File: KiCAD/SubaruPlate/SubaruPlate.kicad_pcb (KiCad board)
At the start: 2 copper layers, 140 x 140 mm, 24 parts, among them J1 DF51A-4P-2DSA, J2 B3B-XH-A(LF)(SN), U1 LPS28DFW, U3 MCP2515-xSO, U4 MCP2562-E-SN, U5 XIAO-RP2040-DIP, Y1 8MHz

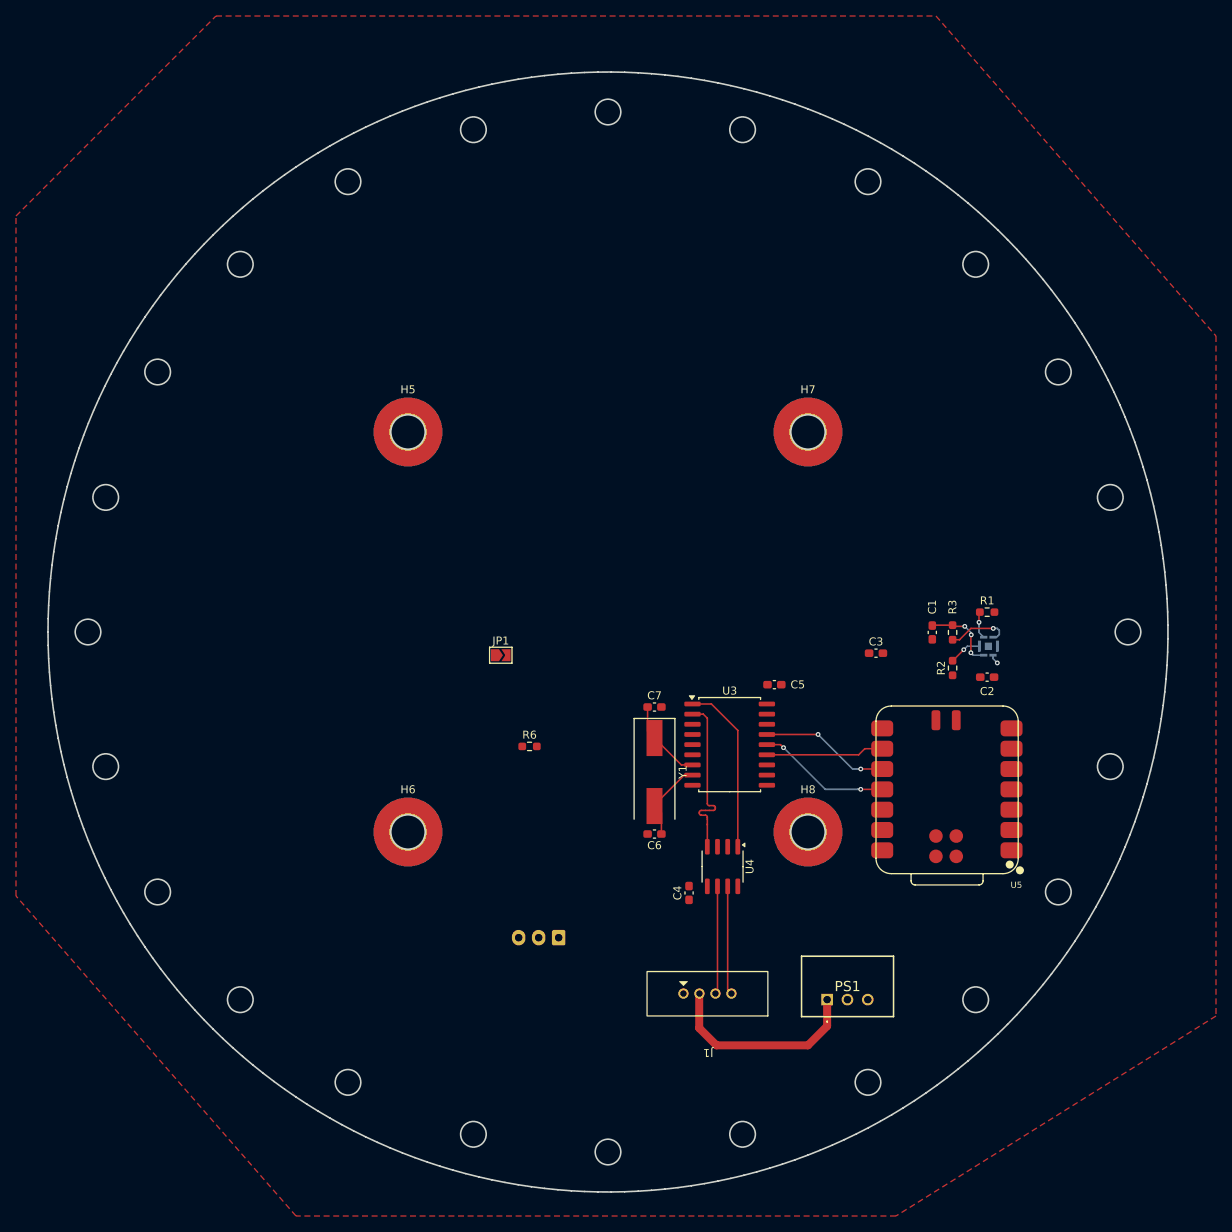
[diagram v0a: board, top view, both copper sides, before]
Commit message: 後は最終確認
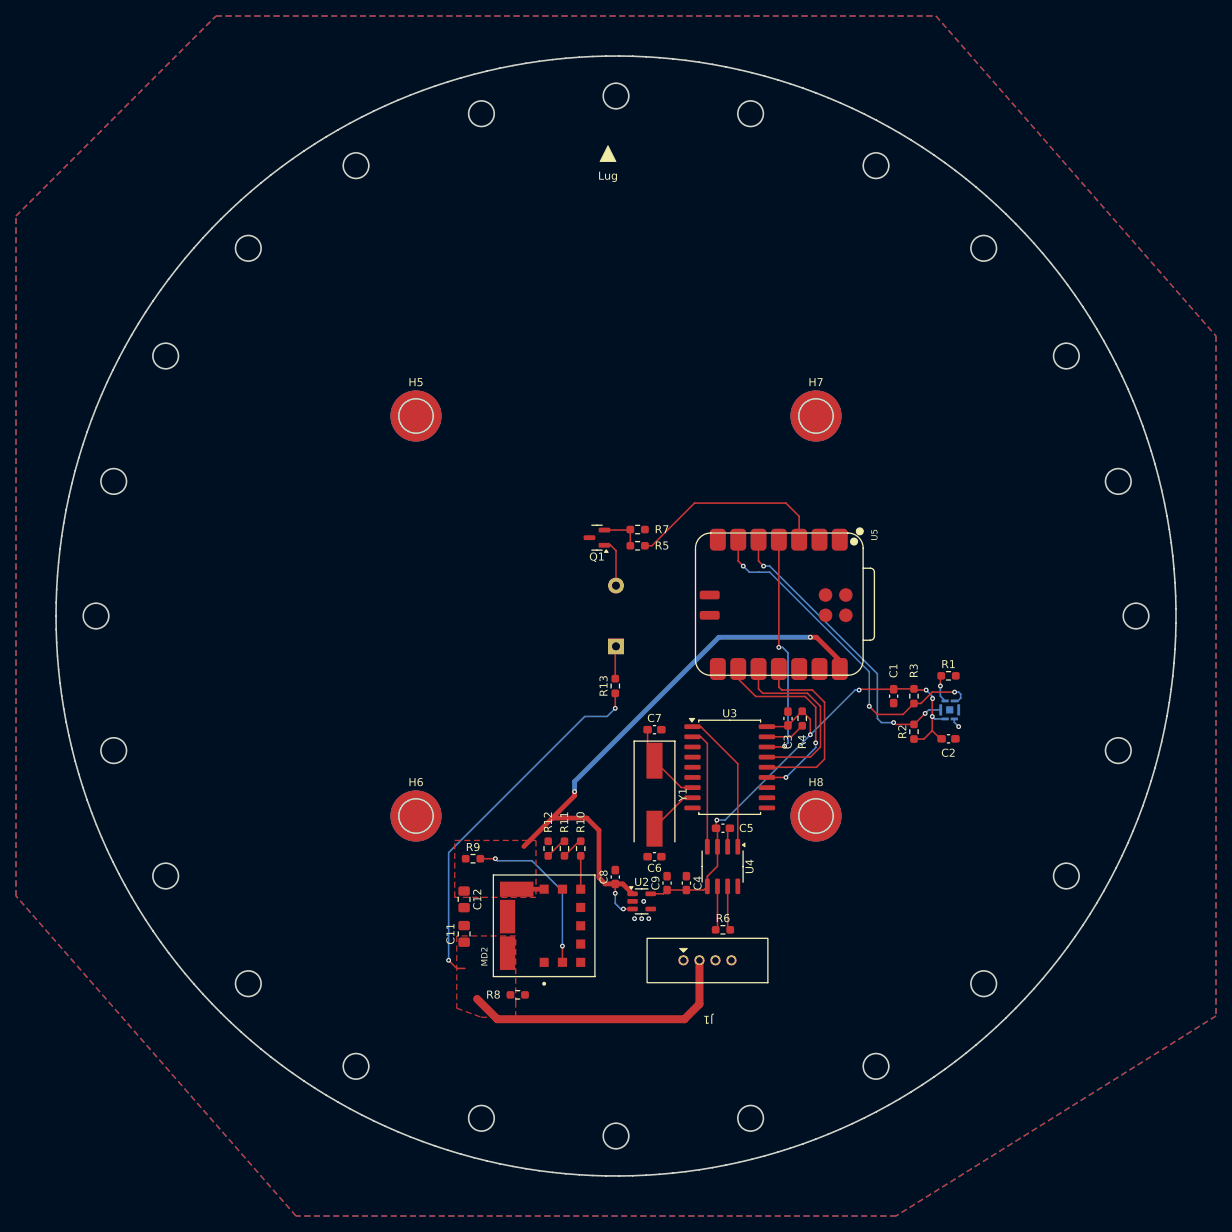
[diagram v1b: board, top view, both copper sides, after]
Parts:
- removed J2: B3B-XH-A(LF)(SN), Connector_JST:JST_XH_B3B-XH-A_1x03_P2.50mm_Vertical
- removed JP1: Jumper_2_Open, Jumper:SolderJumper-2_P1.3mm_Open_TrianglePad1.0x1.5mm
- removed PS1: M78AR05-0.5, TSRP_IC:M78AR03305
- added BZ1: Buzzer, Buzzer_Beeper:Buzzer_12x9.5RM7.6, B.Cu at (150.0, 103.8)
- added C11: 22u, Capacitor_SMD:C_0805_2012Metric_Pad1.18x1.45mm_HandSolder, F.Cu at (131.0, 139.7)
- added C12: 10u, Capacitor_SMD:C_0805_2012Metric_Pad1.18x1.45mm_HandSolder, F.Cu at (131.0, 135.4)
- added C8: 1u, Capacitor_SMD:C_0603_1608Metric_Pad1.08x0.95mm_HandSolder, F.Cu at (149.9, 132.6)
- added C9: 1u, Capacitor_SMD:C_0603_1608Metric_Pad1.08x0.95mm_HandSolder, F.Cu at (156.4, 133.4)
- added MD2: OKL-T_6-W12N-C, TSRP_IC:MURATA_OKL-T-6-W12N-C_0, F.Cu at (141.0, 138.7)
- added Q1: NMOS, Package_TO_SOT_SMD:SOT-23, F.Cu at (147.6, 90.2)
- added R10: 1k 0.1%, Resistor_SMD:R_0603_1608Metric_Pad0.98x0.95mm_HandSolder, F.Cu at (145.6, 129.1)
- added R11: 330 0.1%, Resistor_SMD:R_0603_1608Metric_Pad0.98x0.95mm_HandSolder, F.Cu at (143.6, 129.1)
- added R12: 10 0.1%, Resistor_SMD:R_0603_1608Metric_Pad0.98x0.95mm_HandSolder, F.Cu at (141.5, 129.1)
- added R13: 600, Resistor_SMD:R_0603_1608Metric_Pad0.98x0.95mm_HandSolder, F.Cu at (149.9, 108.8)
- added R4: 10K, Resistor_SMD:R_0603_1608Metric_Pad0.98x0.95mm_HandSolder, F.Cu at (173.3, 112.8)
- added R5: 750, Resistor_SMD:R_0603_1608Metric_Pad0.98x0.95mm_HandSolder, F.Cu at (152.7, 91.2)
- added R7: 10k, Resistor_SMD:R_0603_1608Metric_Pad0.98x0.95mm_HandSolder, F.Cu at (152.7, 89.2)
- added R8: 20k, Resistor_SMD:R_0603_1608Metric_Pad0.98x0.95mm_HandSolder, F.Cu at (137.7, 147.4)
- added R9: 100k, Resistor_SMD:R_0603_1608Metric_Pad0.98x0.95mm_HandSolder, F.Cu at (132.1, 130.3)
- added U2: NCV8114BSN330T1G, Package_TO_SOT_SMD:TSOT-23-5, F.Cu at (153.2, 135.7)
- H5, H6, H7, H8: footprint MountingHole:MountingHole_4.3mm_M4_Pad_TopBottom -> MountingHole:MountingHole_3.2mm_M3_Pad_TopBottom
- moved R6 33.3 mm to (163.4, 139.2)
- moved U5 31.4 mm to (170.4, 98.5), turned to -90 degrees
- moved C5 19.1 mm to (163.4, 126.5)
- moved C3 13.7 mm to (171.5, 112.8), turned to 90 degrees
- moved R1 9.31 mm to (191.6, 107.5)
- moved C1 9.31 mm to (184.7, 110.0)
- moved R2 9.31 mm to (187.2, 114.5)
- moved R3 9.31 mm to (187.2, 110.0)
- moved U1 9.31 mm to (191.7, 111.7)
- moved C2 9.10 mm to (191.6, 115.4)
- moved J1 4.15 mm to (161.4, 140.4)
- moved C6 2.83 mm to (154.8, 130.1)
- moved C7 2.83 mm to (154.8, 114.2)
- moved U3 2.83 mm to (164.2, 118.9)
- moved Y1 2.83 mm to (154.8, 122.3)
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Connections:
- R6 pad 2: Net-(JP1-B) -> CAN_H
- U5 pad 12: +3.3V -> unconnected-(U5-3V3-Pad12)
- U5 pad 3: unconnected-(U5-GPIO28/ADC2/A2-Pad3) -> Buzzer
- U5 pad 4: unconnected-(U5-GPIO29/ADC3/A3-Pad4) -> SPI_CS_MCP2515
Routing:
- net +5V: track 0.00 -> 79.6 mm, vias 0 -> 4
- net +3.3V: track 9.54 -> 69.4 mm, vias 3 -> 6
- net +12V: track 25.5 -> 81.2 mm, vias 0 -> 2
- net I2C_SCL: track 7.98 -> 43.7 mm, vias 1 -> 3
- net I2C_SDA: track 4.10 -> 37.9 mm, vias 1 -> 3
- net SPI_CS_MCP2515: track 0.00 -> 29.0 mm, vias 0 -> 2
- net Buzzer: track 0.00 -> 25.1 mm
- net P.G._OKL-T/6-W12N-C: track 0.00 -> 20.8 mm, vias 0 -> 2
- net SPI_SCK: track 14.7 -> 25.1 mm, vias 0 -> 2
- net CAN_H: track 13.6 -> 5.57 mm
- net CAN_L: track 13.5 -> 5.53 mm
- net SPI_MISO: track 16.2 -> 23.5 mm, vias 2 -> 0
- net SPI_MOSI: track 16.7 -> 23.5 mm, vias 2 -> 0
- net CAN_RX: track 21.5 -> 15.1 mm
- net Net-(BZ1--): track 0.00 -> 6.09 mm
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- added copper zone on F.Cu, net +12V
- added copper zone on F.Cu, net +5V
- added copper zone on B.Cu, net GND
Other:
- outline, holes or cut-outs redrawn
- board text added: "Lug"
